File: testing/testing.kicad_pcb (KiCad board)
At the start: 2 copper layers, 106.8 x 66.8 mm, 0 parts

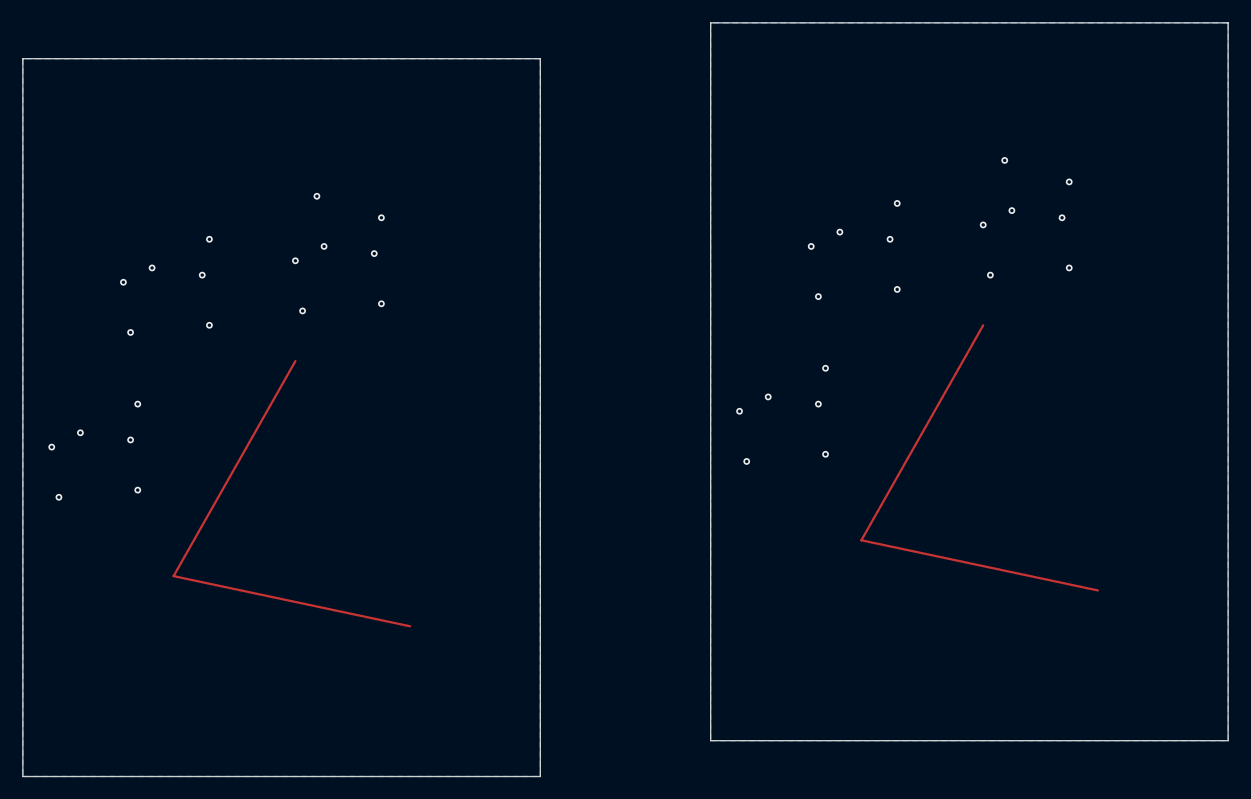
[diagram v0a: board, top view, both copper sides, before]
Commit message: Test Commit 11
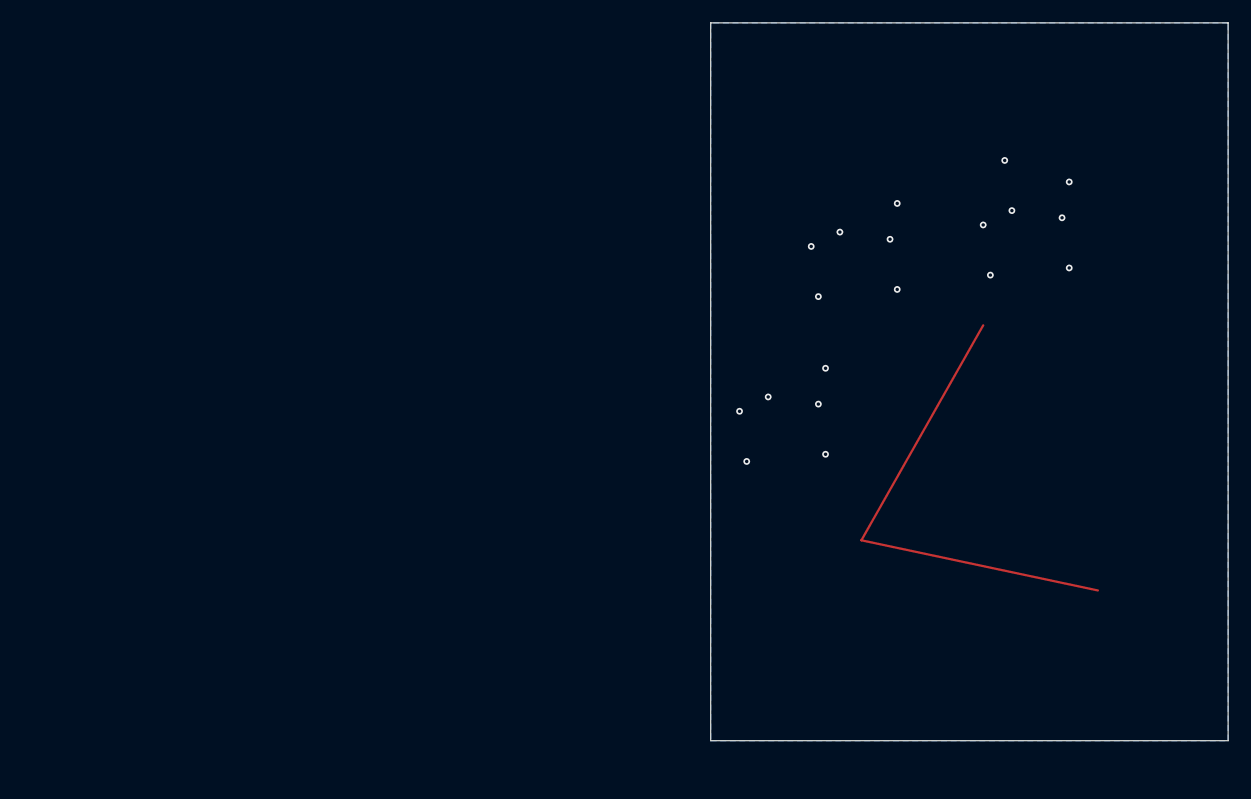
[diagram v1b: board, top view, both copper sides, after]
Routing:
- net (no net): vias 38 -> 19
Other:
- board size 106.8 x 66.8 mm -> 45.8 x 63.6 mm
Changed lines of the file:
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@@
-	)
-	(gr_line
-		(start 85.11 96.52)
-		(end 74.315 115.57)
-		(stroke
-			(width 0.2)
-			(type default)
-		)
-		(layer "F.Cu")
 	)
 	(gr_line
 		(start 146.05 93.345)
 		(end 135.255 112.395)
-		(stroke
-			(width 0.2)
-			(type default)
-		)
-		(layer "F.Cu")
-	)
-	(gr_line
-		(start 74.315 115.57)
-		(end 95.27 120.015)
 		(stroke
 			(width 0.2)
@@
 		(layer "Edge.Cuts")
 	)
-	(gr_rect
-		(start 60.96 69.725)
-		(end 106.81 133.325)
-		(stroke
-			(width 0.05)
-			(type default)
-		)
-		(fill no)
-		(layer "Edge.Cuts")
-	)
 	(via
 		(at 133.35 85.09)
-		(size 0.6)
-		(drill 0.3)
-		(layers "F.Cu" "B.Cu")
-		(net 0)
-	)
-	(via
-		(at 69.87 89.535)
 		(size 0.6)
 		(drill 0.3)
@@
 	)
 	(via
-		(at 71.14 100.33)
-		(size 0.6)
-		(drill 0.3)
-		(layers "F.Cu" "B.Cu")
-		(net 0)
-	)
-	(via
-		(at 66.06 102.87)
-		(size 0.6)
-		(drill 0.3)
-		(layers "F.Cu" "B.Cu")
-		(net 0)
-	)
-	(via
 		(at 125.095 105.41)
 		(size 0.6)
@@
 	)
 	(via
-		(at 72.41 88.265)
-		(size 0.6)
-		(drill 0.3)
-		(layers "F.Cu" "B.Cu")
-		(net 0)
-	)
-	(via
 		(at 138.43 82.55)
-		(size 0.6)
-		(drill 0.3)
-		(layers "F.Cu" "B.Cu")
-		(net 0)
-	)
-	(via
-		(at 85.745 92.075)
-		(size 0.6)
-		(drill 0.3)
-		(layers "F.Cu" "B.Cu")
-		(net 0)
-	)
-	(via
-		(at 87.65 86.36)
 		(size 0.6)
 		(drill 0.3)
@@
 	)
 	(via
-		(at 70.505 93.98)
-		(size 0.6)
-		(drill 0.3)
-		(layers "F.Cu" "B.Cu")
-		(net 0)
-	)
-	(via
 		(at 148.59 83.185)
 		(size 0.6)
@@
 	)
 	(via
-		(at 92.73 83.82)
-		(size 0.6)
-		(drill 0.3)
-		(layers "F.Cu" "B.Cu")
-		(net 0)
-	)
-	(via
-		(at 87.015 81.915)
-		(size 0.6)
-		(drill 0.3)
-		(layers "F.Cu" "B.Cu")
-		(net 0)
-	)
-	(via
 		(at 137.795 85.725)
 		(size 0.6)
@@
 	)
 	(via
-		(at 92.095 86.995)
-		(size 0.6)
-		(drill 0.3)
-		(layers "F.Cu" "B.Cu")
-		(net 0)
-	)
-	(via
-		(at 76.855 88.9)
-		(size 0.6)
-		(drill 0.3)
-		(layers "F.Cu" "B.Cu")
-		(net 0)
-	)
-	(via
-		(at 64.155 108.585)
-		(size 0.6)
-		(drill 0.3)
-		(layers "F.Cu" "B.Cu")
-		(net 0)
-	)
-	(via
-		(at 71.14 107.95)
-		(size 0.6)
-		(drill 0.3)
-		(layers "F.Cu" "B.Cu")
-		(net 0)
-	)
-	(via
-		(at 77.49 85.725)
-		(size 0.6)
-		(drill 0.3)
-		(layers "F.Cu" "B.Cu")
-		(net 0)
-	)
-	(via
-		(at 85.11 87.63)
-		(size 0.6)
-		(drill 0.3)
-		(layers "F.Cu" "B.Cu")
-		(net 0)
-	)
-	(via
 		(at 127 99.695)
-		(size 0.6)
-		(drill 0.3)
-		(layers "F.Cu" "B.Cu")
-		(net 0)
-	)
-	(via
-		(at 77.49 93.345)
-		(size 0.6)
-		(drill 0.3)
-		(layers "F.Cu" "B.Cu")
-		(net 0)
-	)
-	(via
-		(at 70.505 103.505)
-		(size 0.6)
-		(drill 0.3)
-		(layers "F.Cu" "B.Cu")
-		(net 0)
-	)
-	(via
-		(at 63.52 104.14)
-		(size 0.6)
-		(drill 0.3)
-		(layers "F.Cu" "B.Cu")
-		(net 0)
-	)
-	(via
-		(at 92.73 91.44)
 		(size 0.6)
 		(drill 0.3)
@@
 			)
 		)
-	)
-	(zone
-		(net 0)
-		(net_name "")
-		(layer "B.Cu")
-		(hatch edge 0.5)
-		(connect_pads
-			(clearance 0.5)
-		)
-		(min_thickness 0.25)
-		(filled_areas_thickness no)
-		(fill yes
-			(thermal_gap 0.5)
-			(thermal_bridge_width 0.5)
-			(island_removal_mode 1)
-			(island_area_min 10)
-		)
-		(polygon
-			(pts
-				(xy 60.96 69.725) (xy 60.96 133.325) (xy 106.81 133.325) (xy 106.81 69.725)
-			)
-		)
